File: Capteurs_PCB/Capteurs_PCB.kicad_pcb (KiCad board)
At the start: 2 copper layers, 89 x 72 mm, 56 parts, among them J1 Conn_01x04, J101 Conn_01x03, J103 Conn_02x20_Odd_Even, J104 Conn_ST_STDC14, J2 Conn_01x03, J3 Alim_Prop2, J4 Conn_01x02, J5 Alim_Prop1, J6 Conn_01x03, J7 Conn_01x03, SW101 SW_DPDT_x2, U1 STM32L412KBTx, U3 LSM6DSL, U6 32350268

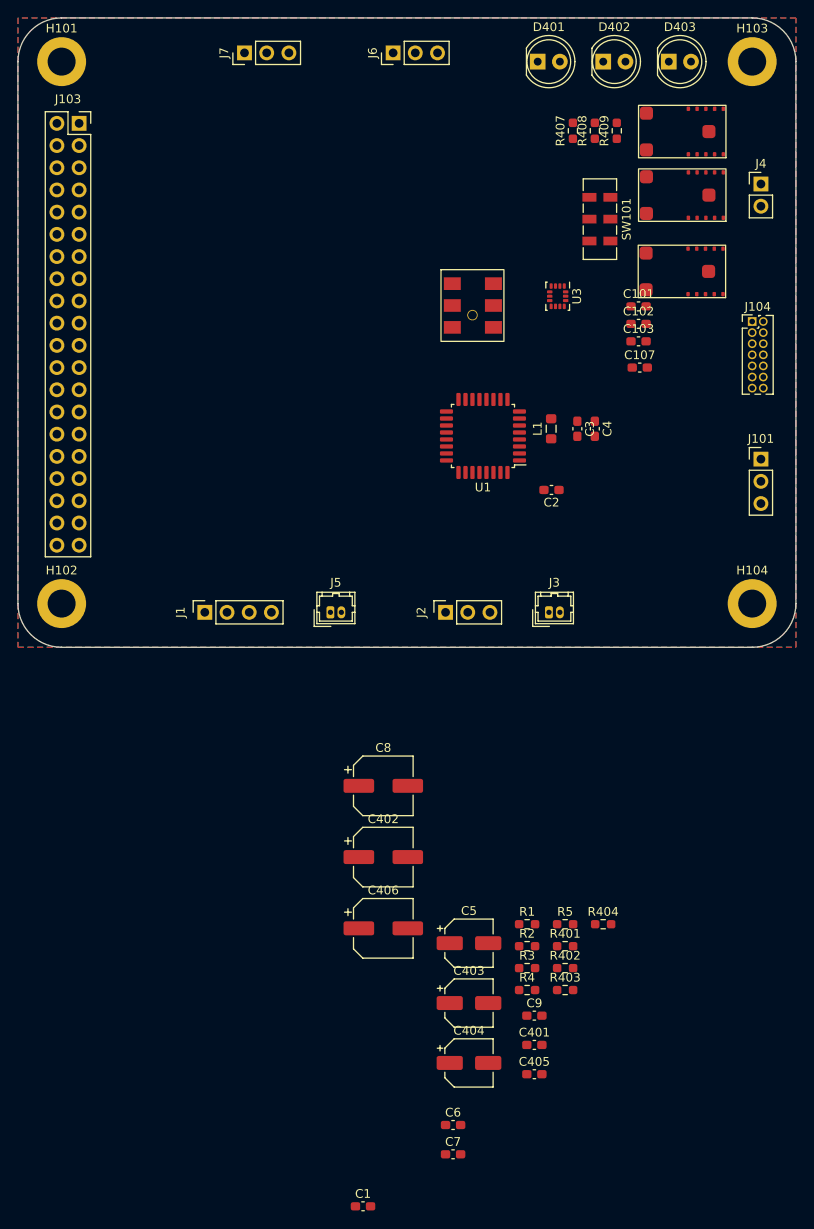
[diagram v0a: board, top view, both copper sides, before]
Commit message: Suite
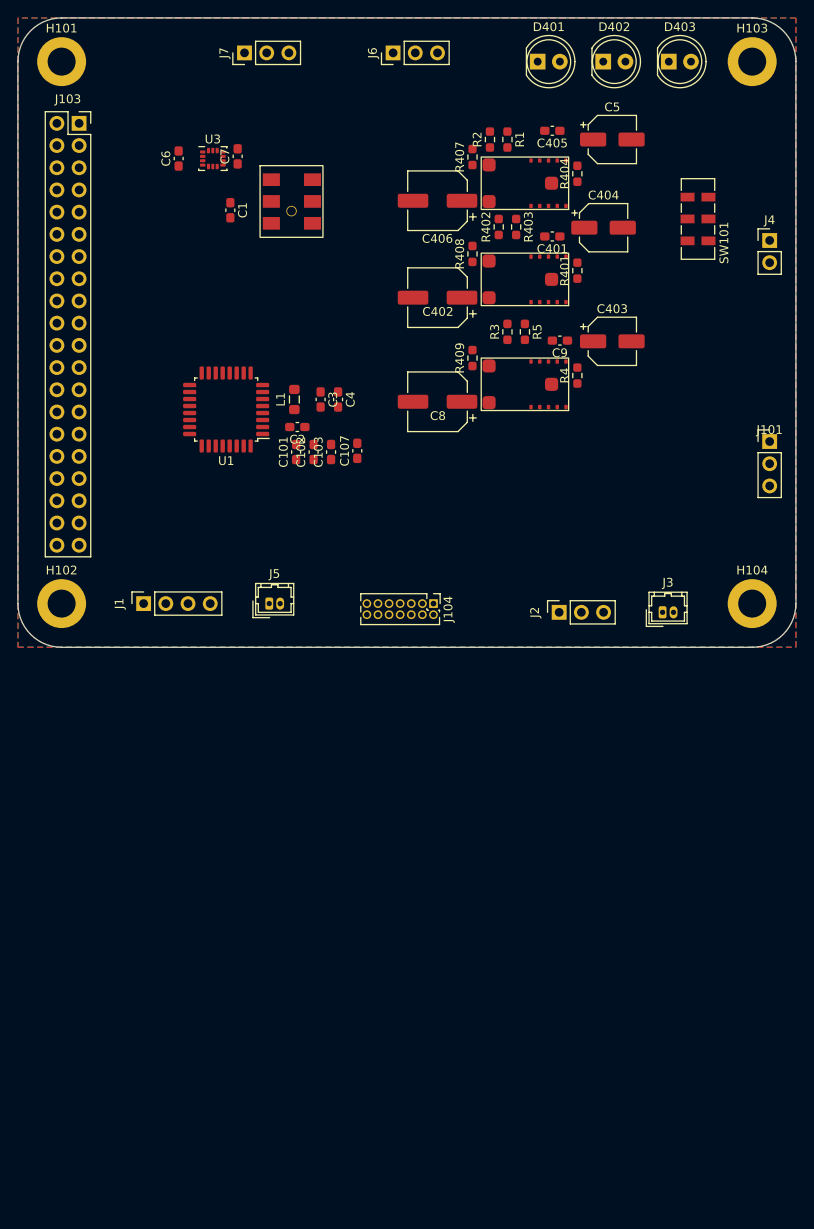
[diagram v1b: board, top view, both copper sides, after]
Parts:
- moved C7 116.8 mm to (98.1, 71.8), turned to 90 degrees
- moved C1 115.0 mm to (97.3, 78.0), turned to -90 degrees
- moved C6 114.9 mm to (91.4, 72.1), turned to 90 degrees
- moved C405 107.9 mm to (134.1, 68.9), turned to 180 degrees
- moved C404 96.8 mm to (140.0, 80.0)
- moved C5 93.4 mm to (141.0, 69.9)
- moved C401 92.5 mm to (134.1, 81.0), turned to 180 degrees
- moved R2 92.4 mm to (127.0, 69.9), turned to 90 degrees
- moved R1 89.8 mm to (129.0, 69.9), turned to -90 degrees
- moved R403 87.5 mm to (130.0, 79.9), turned to -90 degrees
- moved R404 85.9 mm to (137.0, 73.8), turned to 90 degrees
- moved R402 85.1 mm to (128.0, 79.9), turned to 90 degrees
- moved C406 83.5 mm to (121.0, 76.9), turned to 180 degrees
- moved C403 77.5 mm to (141.0, 93.0)
- moved R401 77.3 mm to (137.0, 84.9), turned to 90 degrees
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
